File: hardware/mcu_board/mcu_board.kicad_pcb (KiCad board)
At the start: 2 copper layers, 57.9 x 100 mm, 17 parts, among them J1 TEMP, J3 LEDS_IN, J4 DISPLAY, J5 RTC, J6 MCU, J8 LEDS_OUT, SW1 RESET, SW2 RotaryEncoder_Switch, U1 ESP32-S3-DevKitC

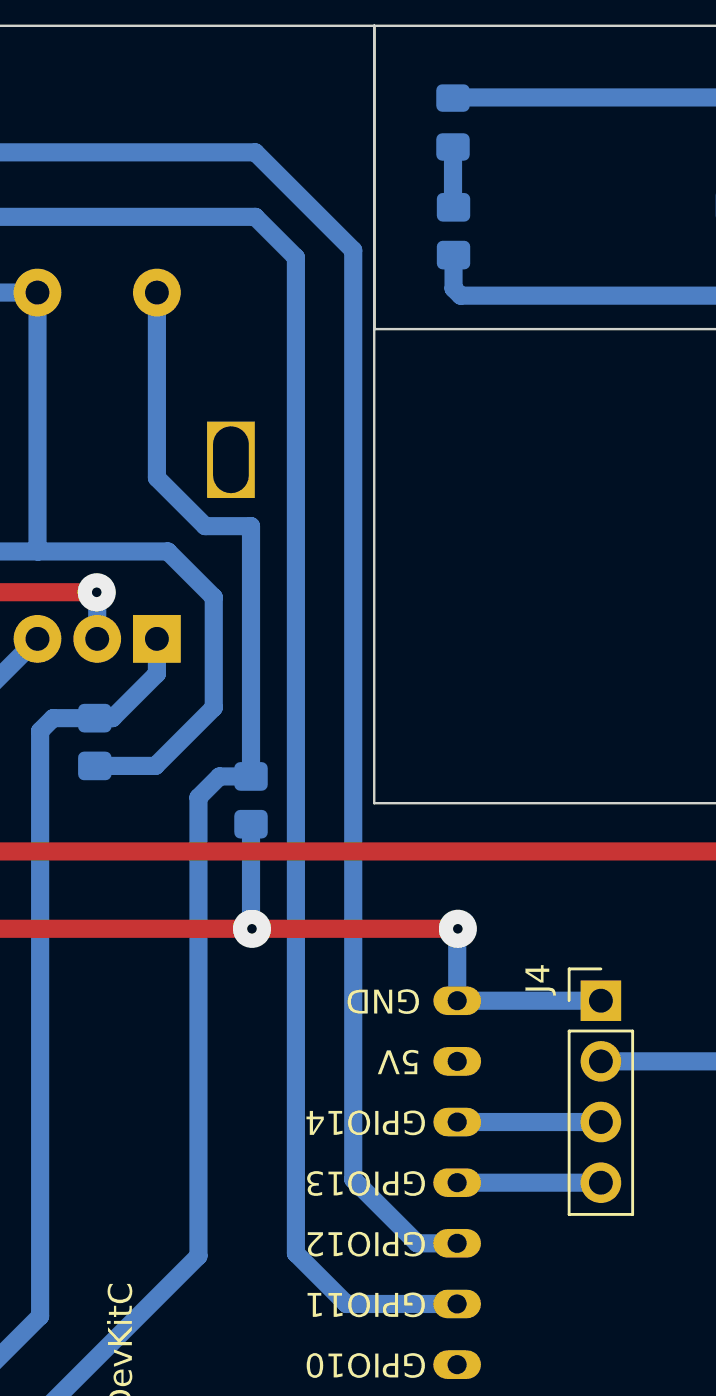
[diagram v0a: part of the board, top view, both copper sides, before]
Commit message: move screw position
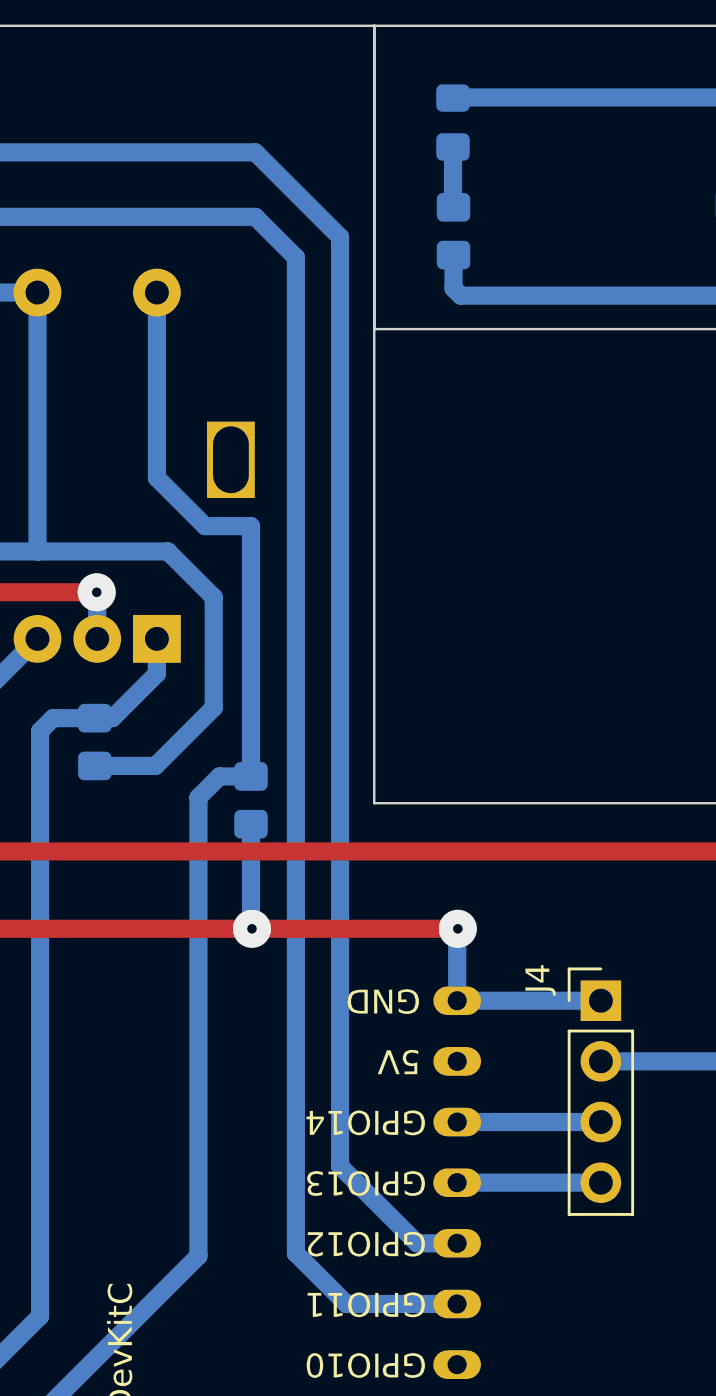
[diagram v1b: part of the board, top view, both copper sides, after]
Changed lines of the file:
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@@
     (pcbplotparams
       (layerselection 0x0001000_7ffffffe)
-      (plot_on_all_layers_selection 0x0001000_80000000)
+      (plot_on_all_layers_selection 0x003df30_80000001)
       (disableapertmacros false)
       (usegerberextensions false)
@@
       (dxfimperialunits false)
       (dxfusepcbnewfont true)
-      (psnegative true)
+      (psnegative false)
       (psa4output false)
       (plotreference true)
@@
       (subtractmaskfromsilk false)
       (outputformat 5)
-      (mirror false)
+      (mirror true)
       (drillshape 1)
       (scaleselection 1)
@@
     (fp_line (start 1 0.625) (end 1 -0.625)
       (stroke (width 0.1) (type solid)) (layer "B.Fab"))
-    (pad "1" smd roundrect (at -1 0 270) (size 1.2 1.4) (layers "B.Cu" "B.Paste" "B.Mask") (roundrect_rratio 0.208333)
+    (pad "1" smd roundrect (at -1 0 270) (size 1.2 1.4) (layers "B.Cu" "B.Paste" "B.Mask") (roundrect_rratio 0.2083333333)
       (net 48 "Net-(D2-A)") (pintype "passive"))
-    (pad "2" smd roundrect (at 1 0 270) (size 1.2 1.4) (layers "B.Cu" "B.Paste" "B.Mask") (roundrect_rratio 0.208333)
+    (pad "2" smd roundrect (at 1 0 270) (size 1.2 1.4) (layers "B.Cu" "B.Paste" "B.Mask") (roundrect_rratio 0.2083333333)
       (net 47 "Net-(J3-Pin_3)") (pintype "passive"))
     (model "${KICAD6_3DMODEL_DIR}/Resistor_SMD.3dshapes/R_0805_2012Metric.wrl"
@@
   (segment (start 68.6 41.32) (end 68.6 40.8) (width 0.76) (layer "B.Cu") (net 31))
   (segment (start 68.6 40.8) (end 70.64 38.76) (width 0.76) (layer "B.Cu") (net 31))
-  (segment (start 92.3 45.4) (end 88.2 41.3) (width 0.76) (layer "B.Cu") (net 32))
-  (segment (start 94.97844 86.97844) (end 92.3 84.3) (width 0.76) (layer "B.Cu") (net 32))
-  (segment (start 92.3 84.3) (end 92.3 45.4) (width 0.76) (layer "B.Cu") (net 32))
+  (segment (start 94.97844 86.97844) (end 91.75 83.75) (width 0.76) (layer "B.Cu") (net 32))
+  (segment (start 91.75 83.75) (end 91.75 44.85) (width 0.76) (layer "B.Cu") (net 32))
+  (segment (start 91.75 44.85) (end 88.2 41.3) (width 0.76) (layer "B.Cu") (net 32))
+  (segment (start 88.2 41.3) (end 72.3 41.3) (width 0.76) (layer "B.Cu") (net 32))
   (segment (start 96.650001 86.97844) (end 94.97844 86.97844) (width 0.76) (layer "B.Cu") (net 32))
-  (segment (start 88.2 41.3) (end 72.3 41.3) (width 0.76) (layer "B.Cu") (net 32))
   (segment (start 108.0775 43.525) (end 108.0775 42.4225) (width 0.76) (layer "B.Cu") (net 33))
   (segment (start 109.45 41.05) (end 110.0775 41.05) (width 0.76) (layer "B.Cu") (net 33))

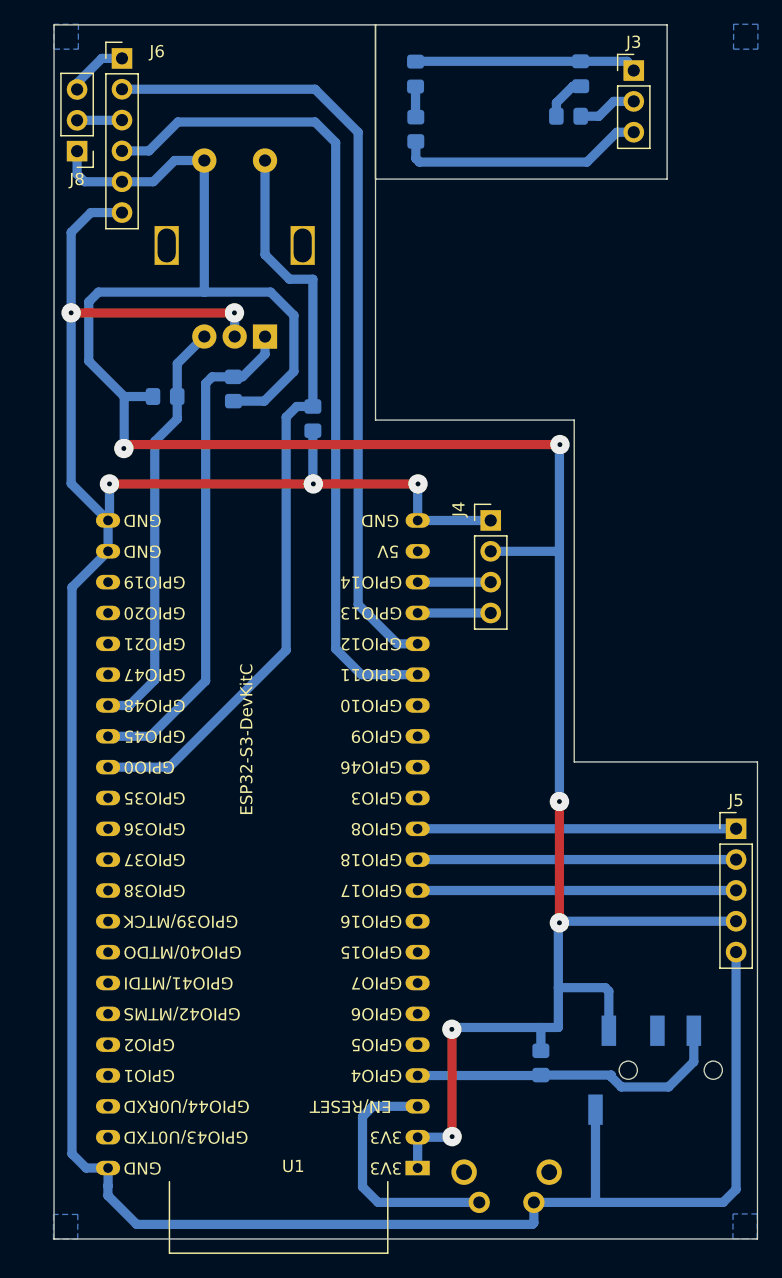
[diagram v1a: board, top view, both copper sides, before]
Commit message: minor tweaks
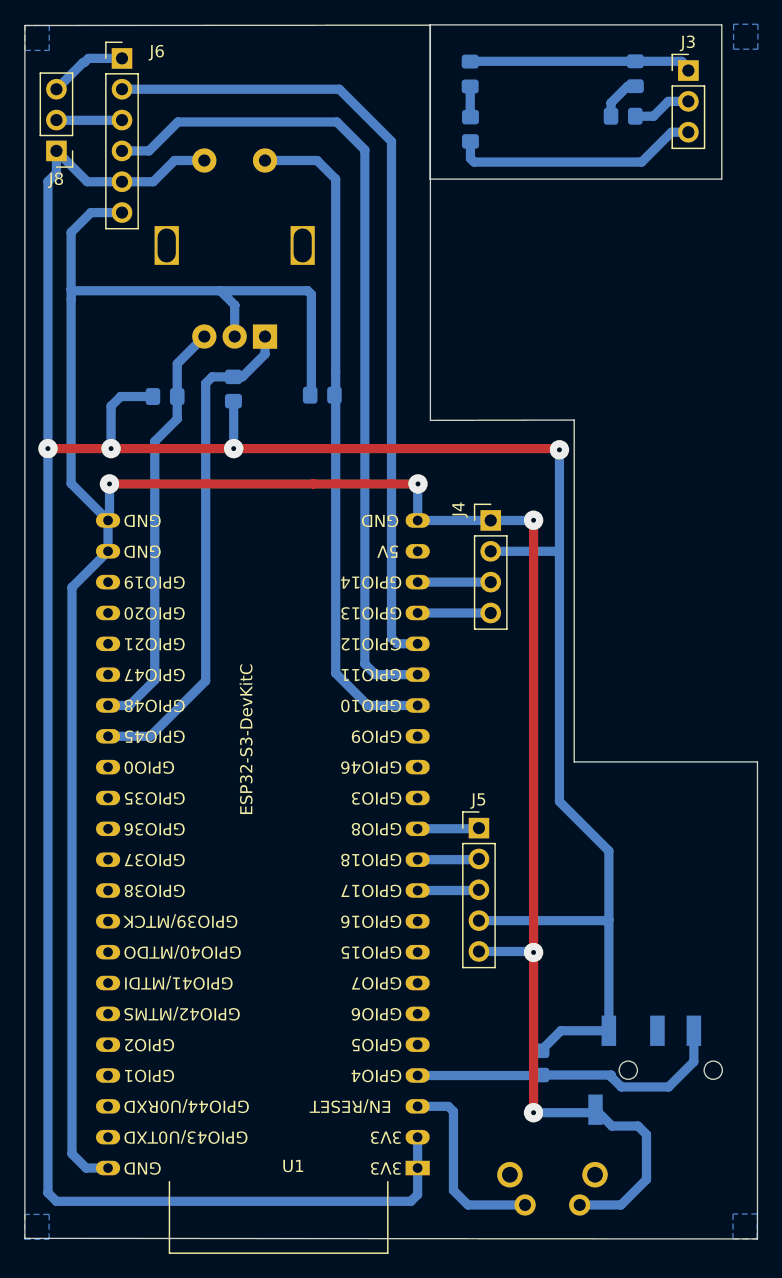
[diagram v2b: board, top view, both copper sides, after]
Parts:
- moved J5 21.2 mm to (101.7, 102.2)
- moved D1 4.50 mm to (114.6, 40.0)
- moved D2 4.50 mm to (101.0, 40.0)
- moved J3 4.50 mm to (119.0, 39.8)
- moved R6 4.50 mm to (113.6, 43.5)
- moved R7 4.50 mm to (101.0, 44.6)
- moved SW1 3.78 mm to (105.5, 133.2)
- moved R5 2.08 mm to (88.8, 66.5), turned to 180 degrees
- moved J8 1.70 mm to (66.9, 46.4)
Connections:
- U1 pad 16: unconnected-(U1-GPIO10/ADC1_CH9-Pad16) -> ROT_SW
- U1 pad 31: ROT_SW -> unconnected-(U1-GPIO0-Pad31)
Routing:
- net +3.3V: track 205.7 -> 262.1 mm, vias 6 -> 4
- net RTC_SDA: track 26.2 -> 4.15 mm
- net RTC_SQW: track 26.2 -> 4.15 mm
- net RTC_SCK: track 26.2 -> 4.17 mm
- net ROT_SW: track 63.5 -> 55.0 mm
- net GND: track 228.4 -> 234.0 mm
- net RESET: track 20.8 -> 16.0 mm
- net LED_BOOST: track 3.71 -> 5.42 mm
- net LED_OFFPEAK: track 5.06 -> 6.45 mm
- net RELAY_OFFPEAK: track 66.1 -> 67.2 mm
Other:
- board size 57.9 x 100 mm -> 60.3 x 100 mm
